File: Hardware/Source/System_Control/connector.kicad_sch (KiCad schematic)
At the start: 35 parts, among them J10 BAL_BAT_CONN2, J11 NTC_CONN, J12 NTC_CONN, J3 SIGNAL_CONN, J4 Conn_01x02_Socket, J5 FLASH_CONN, J6 Conn_01x02_Socket, J7 NTC_CONN, J8 NTC_CONN, J9 BAL_BAT_CONN1

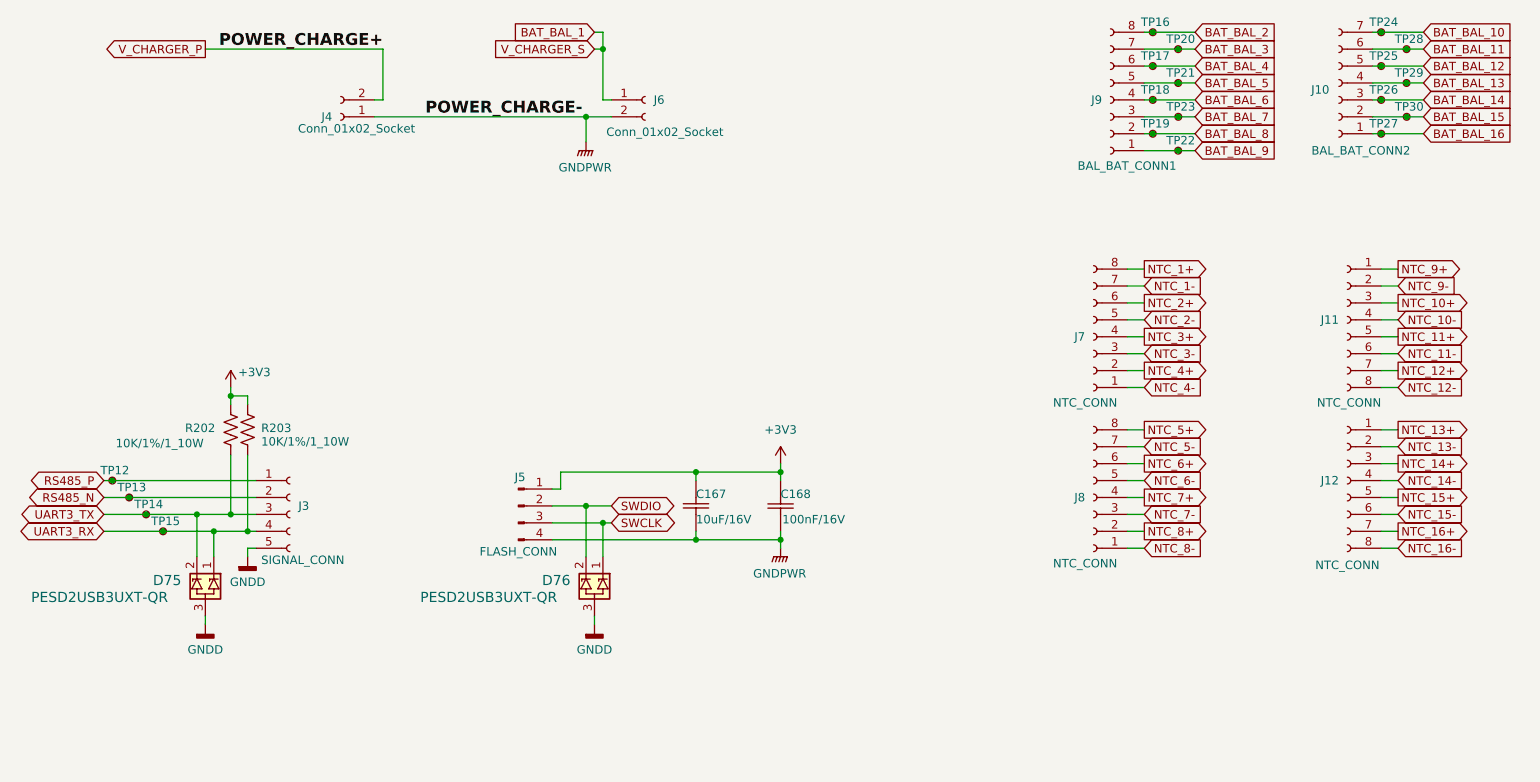
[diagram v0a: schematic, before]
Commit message: check
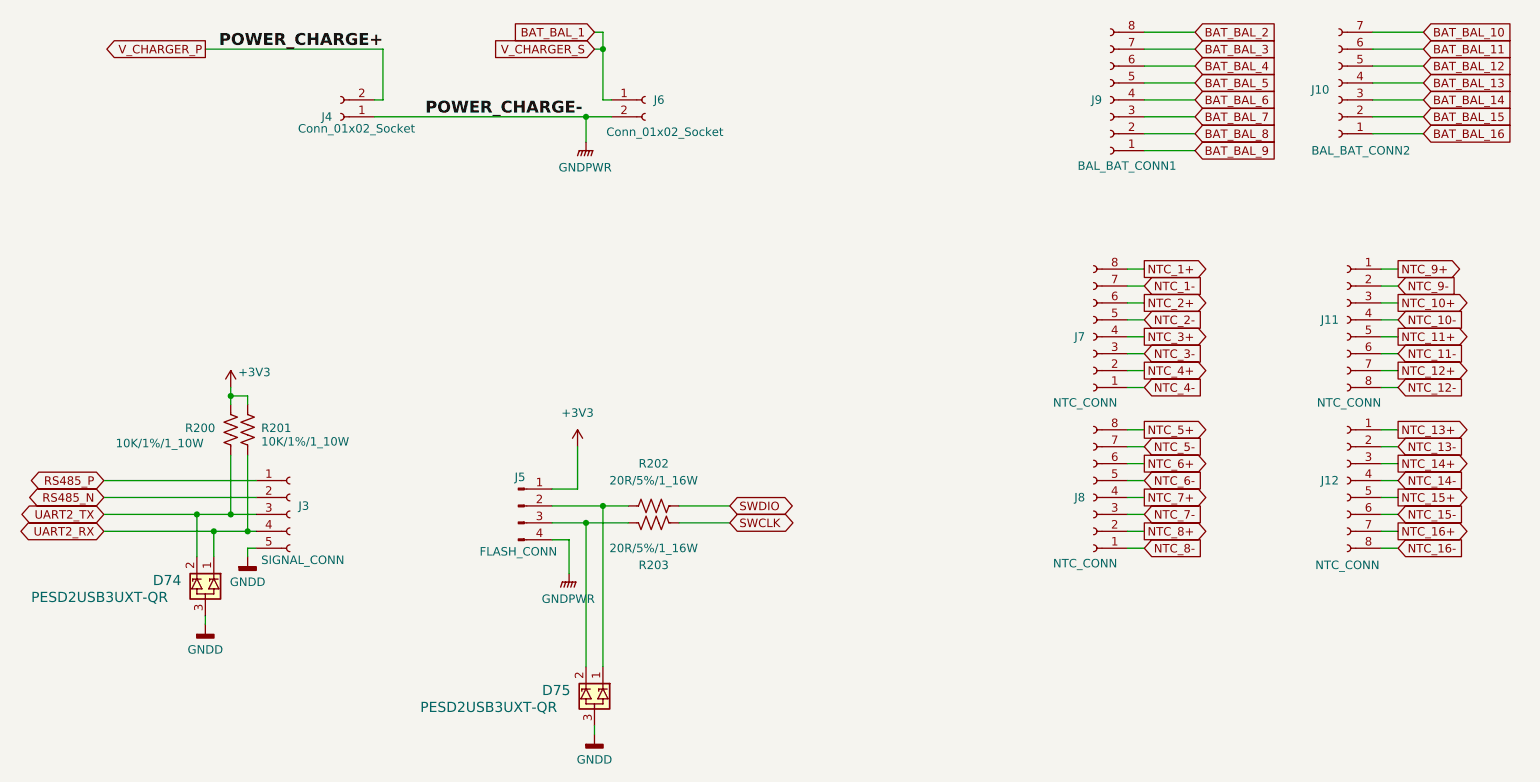
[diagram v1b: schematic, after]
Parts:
- removed C167: 10uF/16V, charge_battery_footprint_lib:Ceramic_Cap_0603, symbol charge_battery_sym_lib:Ceramic_Cap_SMD_10uF_16V
- removed C168: 100nF/16V, charge_battery_footprint_lib:Ceramic_Cap_0603, symbol charge_battery_sym_lib:Ceramic_Cap_SMD_100nF_16V
- removed TP12, TP13, TP14, TP15, TP16, TP17, TP18, TP19, TP20, TP21, TP22, TP23, TP24, TP25, TP26, TP27, TP28, TP29, TP30: TestPoint_Small, TestPoint:TestPoint_Pad_D1.0mm, symbol Connector:TestPoint_Small
- added R202, R203: 20R/5%/1_16W, charge_battery_footprint_lib:Res_0402, symbol charge_battery_sym_lib:Res_20R_0402_5%
- renumbered D75 to D74, D76 to D75, R202 to R200, R203 to R201
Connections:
- net SWCLK: now also R203.2; no longer D75.1, J5.3 (Pin_3)
- net SWDIO: now also R202.2; no longer D75.2, J5.2 (Pin_2)
- net UART3_RX renamed UART2_RX
- net UART3_TX renamed UART2_TX
- new net: D75.1, J5.2 (Pin_2), R202.1
- new net: D75.2, J5.3 (Pin_3), R203.1
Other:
- moved on the sheet: D75
